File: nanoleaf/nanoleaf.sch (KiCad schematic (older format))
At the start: 29 parts, among them J1 Bootloader, J2 Conn_01x04_Male, J3 Conn_01x04_Male, J4 Conn_01x04_Male, U1 ATtiny85-20SU

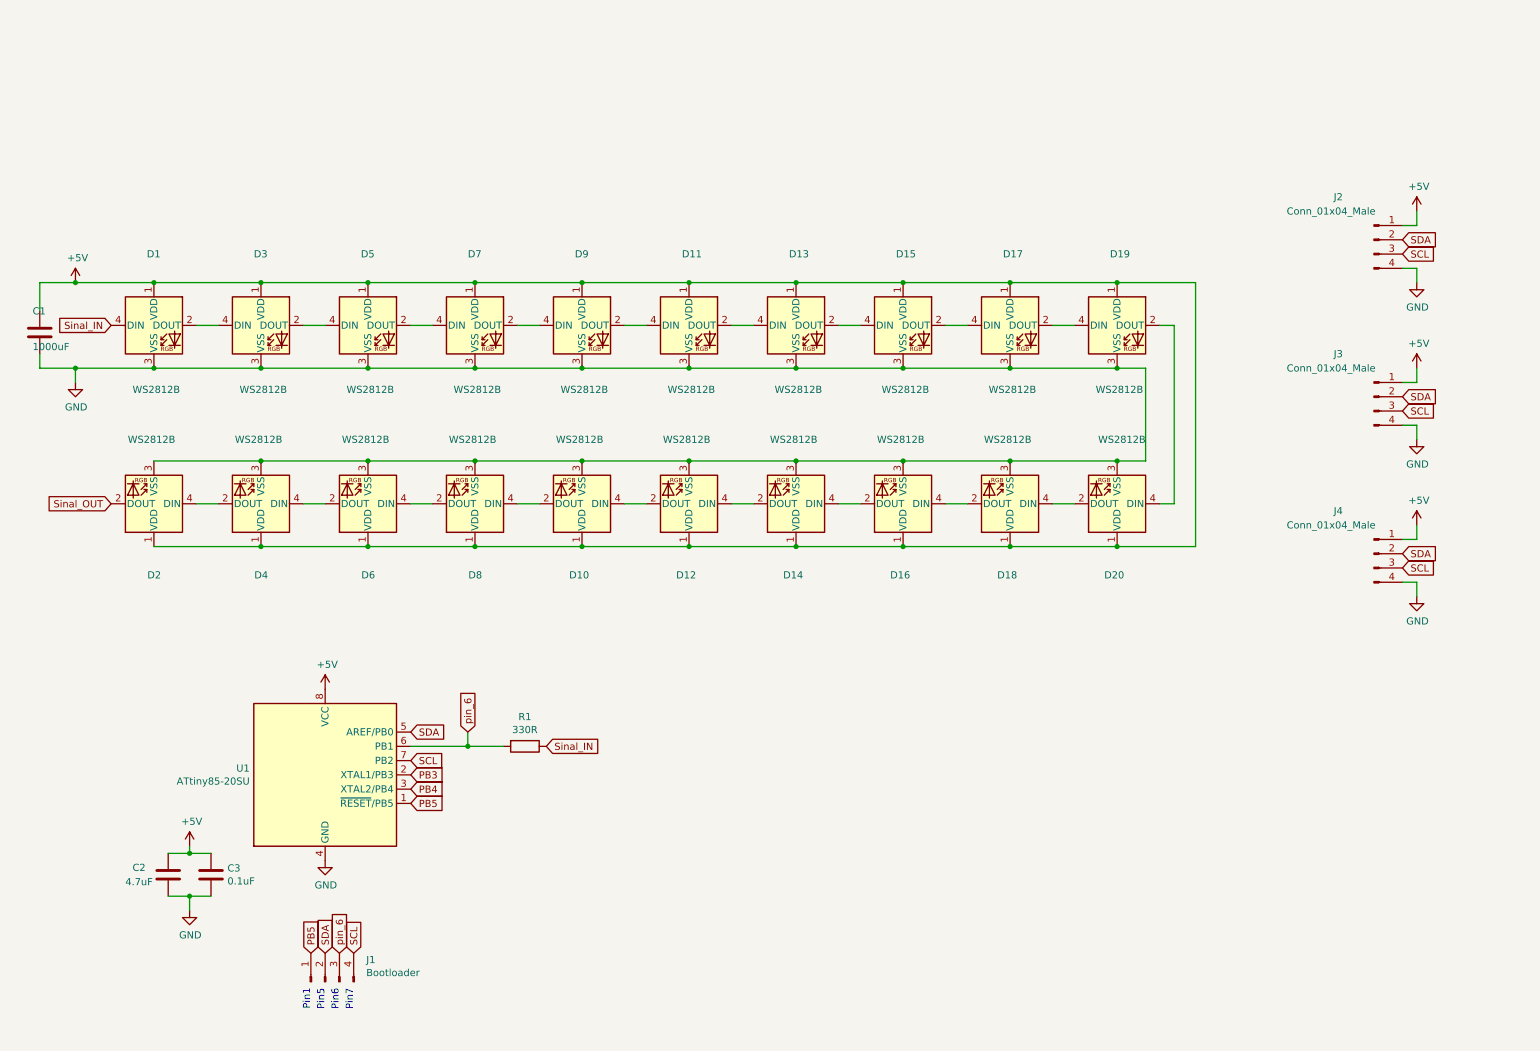
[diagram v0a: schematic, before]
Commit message: Atualização do micro na pcb
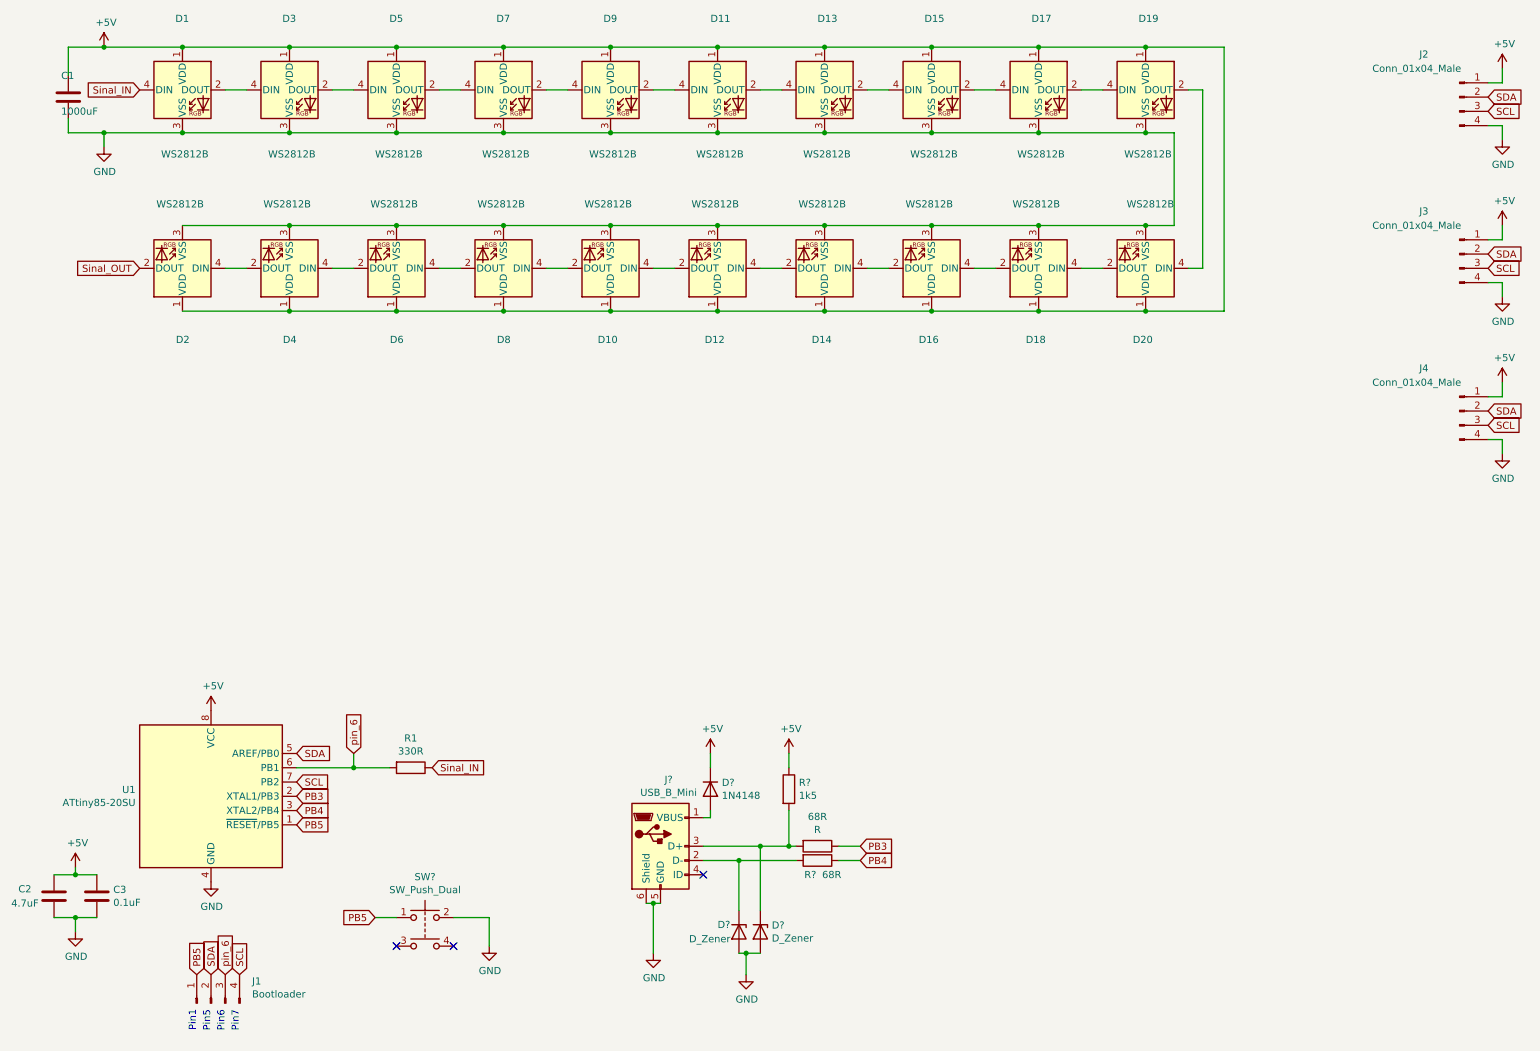
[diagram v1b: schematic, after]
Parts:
- added 68R: R, symbol Device:R
- added D?: 1N4148, symbol Device:D
- added D? (x2): D_Zener, symbol Device:D_Zener
- added J?: USB_B_Mini, symbol Connector:USB_B_Mini
- added R?: 1k5, symbol Device:R
- added R?: 68R, symbol Device:R
- added SW?: SW_Push_Dual, symbol Switch:SW_Push_Dual
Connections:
- net +5V: now also D?.1 (K), R?.1
- net GND: now also D?.2 (A), D?.2 (A), J?.5 (GND), J?.6 (Shield), SW?.2
- net PB3: now also 68R.1
- net PB4: now also R?.1
- net PB5: now also SW?.1
- new net: D?.2 (A), J?.1 (VBUS)
- new net: D?.1 (K), J?.2 (D-), R?.2
- new net: 68R.2, D?.1 (K), J?.3 (D+), R?.2
- no-connect marks 0 -> 3
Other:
- moved on the sheet: C1, C2, C3, D1, D10, D11, D12, D13, D14, D15, D16, D17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
